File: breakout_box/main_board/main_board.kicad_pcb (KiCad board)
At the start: 2 copper layers, 56 x 120 mm, 46 parts, among them CN1 19PIN_LEMO, Q1 DMP3099L, Q2 MJD122, Q3 MMBT5401, Q4 DMP3099L

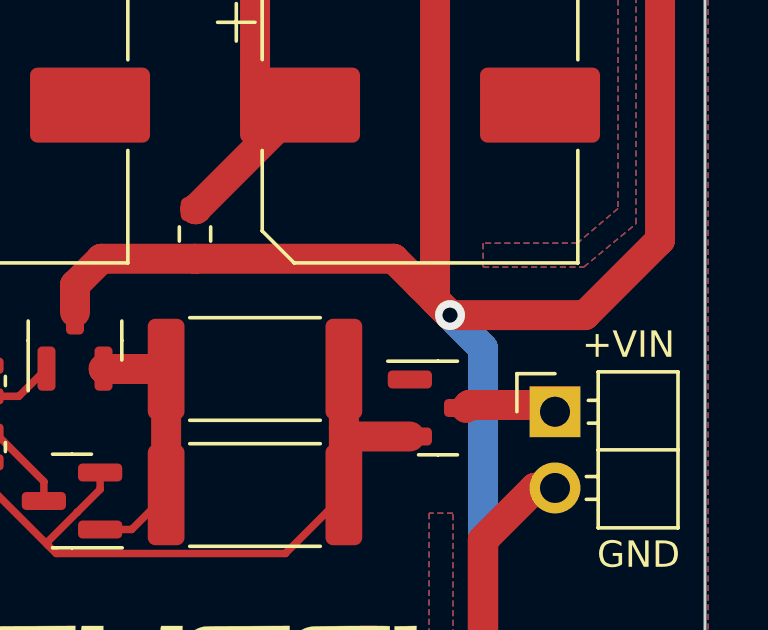
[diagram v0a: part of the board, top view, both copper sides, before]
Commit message: some tweaks
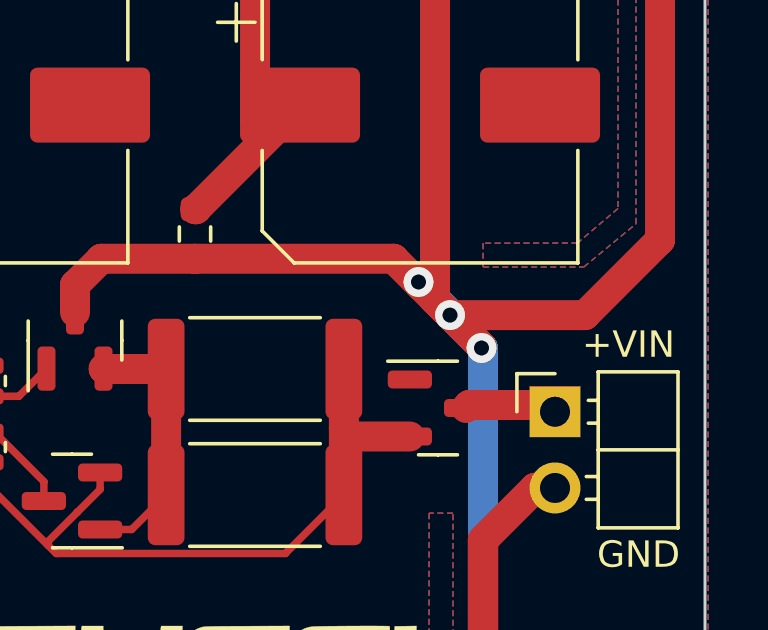
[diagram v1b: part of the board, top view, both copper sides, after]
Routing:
- net V_AUX: track 201.1 -> 204.2 mm, vias 1 -> 3
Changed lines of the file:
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@@
   (segment (start 171.4111 111.0936) (end 170.5011 112.0036) (width 1) (layer "F.Cu") (net 18))
   (segment (start 167.5011 131.0036) (end 167.5011 148.0036) (width 1) (layer "F.Cu") (net 18))
+  (segment (start 169.05 149.6) (end 169.05 149.5525) (width 1) (layer "F.Cu") (net 18))
   (segment (start 155.5 147.5) (end 156.375 146.625) (width 1) (layer "F.Cu") (net 18))
   (segment (start 153.5011 122.0036) (end 151.775 120.2775) (width 0.8) (layer "F.Cu") (net 18))
@@
   (segment (start 175.0011 126.0036) (end 175.0011 146.0036) (width 1) (layer "F.Cu") (net 18))
   (segment (start 170.5011 112.0036) (end 170.5011 124.5036) (width 1) (layer "F.Cu") (net 18))
+  (segment (start 169.05 149.5525) (end 168.0011 148.5036) (width 1) (layer "F.Cu") (net 18))
   (segment (start 167.5011 148.0036) (end 168.0011 148.5036) (width 1) (layer "F.Cu") (net 18))
   (segment (start 170.5011 124.5036) (end 171.0011 125.0036) (width 1) (layer "F.Cu") (net 18))
   (segment (start 156.375 146.625) (end 159.5 146.625) (width 1) (layer "F.Cu") (net 18))
+  (via (at 166.95 147.4) (size 1) (drill 0.5) (layers "F.Cu" "B.Cu") (net 18))
   (via (at 168.0011 148.5036) (size 1) (drill 0.5) (layers "F.Cu" "B.Cu") (net 18))
+  (via (at 169.05 149.6) (size 1) (drill 0.5) (layers "F.Cu" "B.Cu") (net 18))
   (segment (start 124.0011 145.0036) (end 122.2511 145.0036) (width 1) (layer "B.Cu") (net 18))
   (segment (start 124.8975 164.15) (end 166.25 164.15) (width 1) (layer "B.Cu") (net 18))
+  (segment (start 168.0011 148.4511) (end 166.95 147.4) (width 1) (layer "B.Cu") (net 18))
   (segment (start 122.0011 161.2536) (end 124.8975 164.15) (width 1) (layer "B.Cu") (net 18))
   (segment (start 169.1 161.3) (end 169.1 149.6025) (width 1) (layer "B.Cu") (net 18))
@@
   (segment (start 169.1 149.6025) (end 168.0011 148.5036) (width 1) (layer "B.Cu") (net 18))
   (segment (start 124.0011 142.0036) (end 124.0011 145.0036) (width 1) (layer "B.Cu") (net 18))
+  (segment (start 168.0011 148.5036) (end 168.0011 148.4511) (width 1) (layer "B.Cu") (net 18))
   (segment (start 166.25 164.15) (end 169.1 161.3) (width 1) (layer "B.Cu") (net 18))
   (segment (start 140.1011 117.6036) (end 139.2011 118.5036) (width 0.254) (layer "F.Cu") (net 19))
